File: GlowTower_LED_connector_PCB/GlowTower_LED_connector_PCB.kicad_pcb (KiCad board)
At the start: 2 copper layers, 27 x 27 mm, 8 parts, among them U1 LED strip, U2 LED strip, U3 LED strip, U4 LED strip

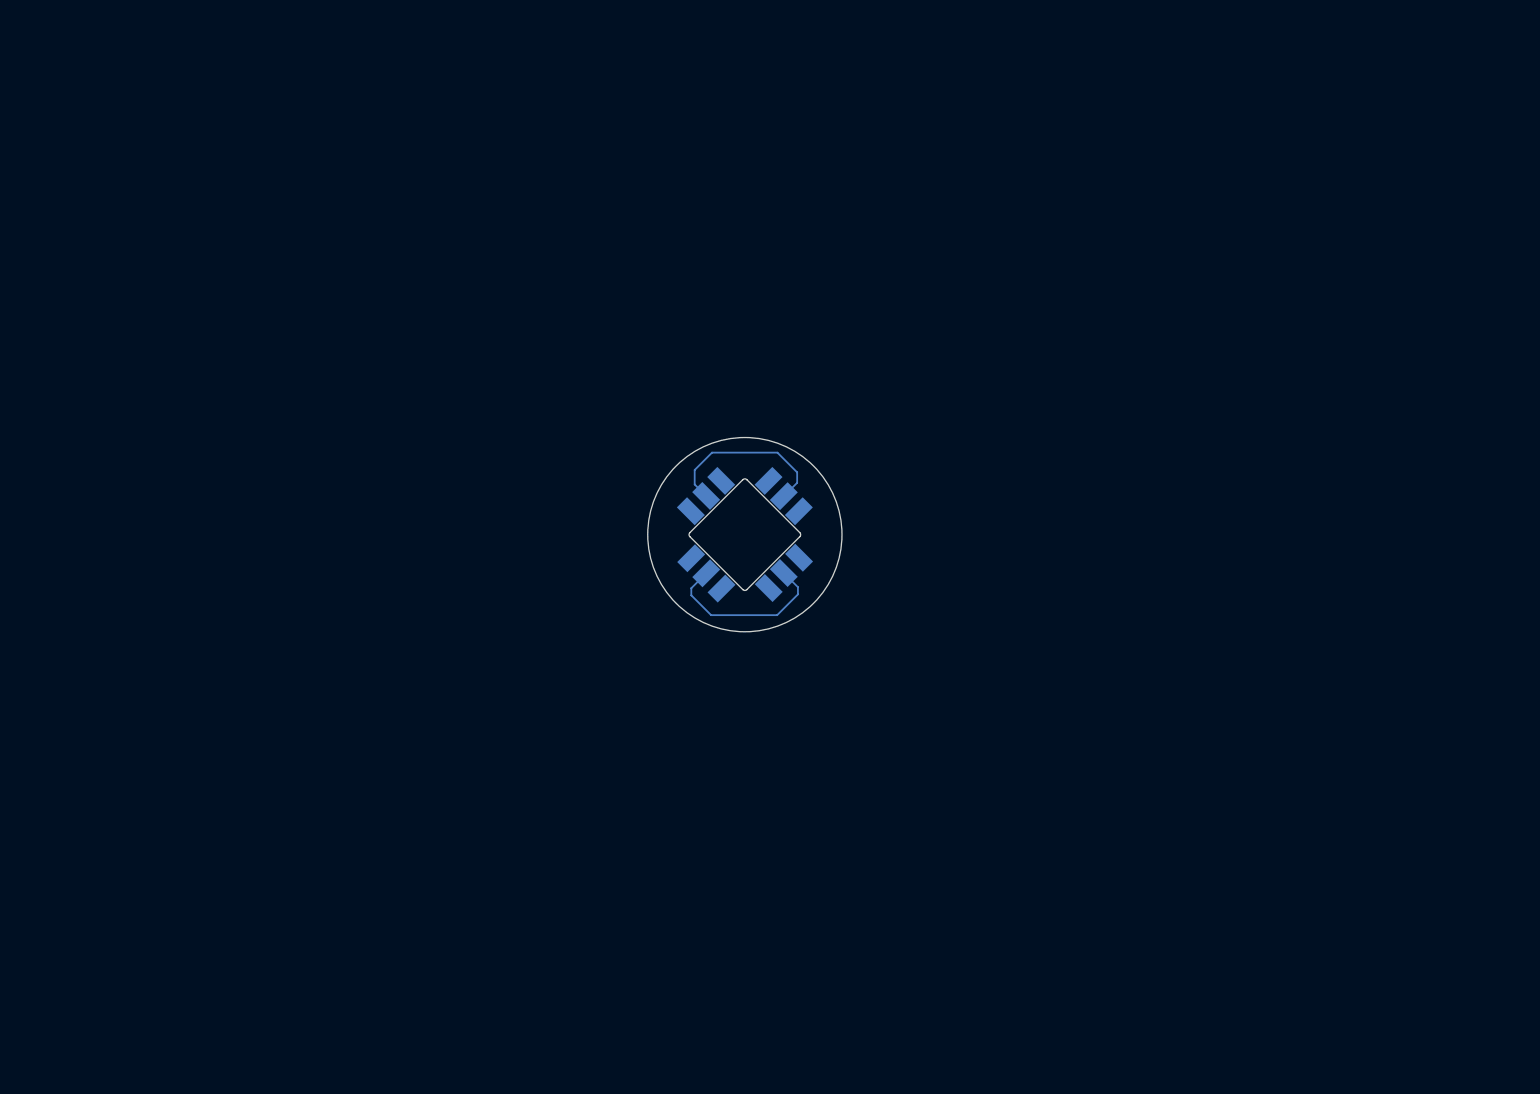
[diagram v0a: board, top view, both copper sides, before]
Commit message: updated pcb design (in progress)
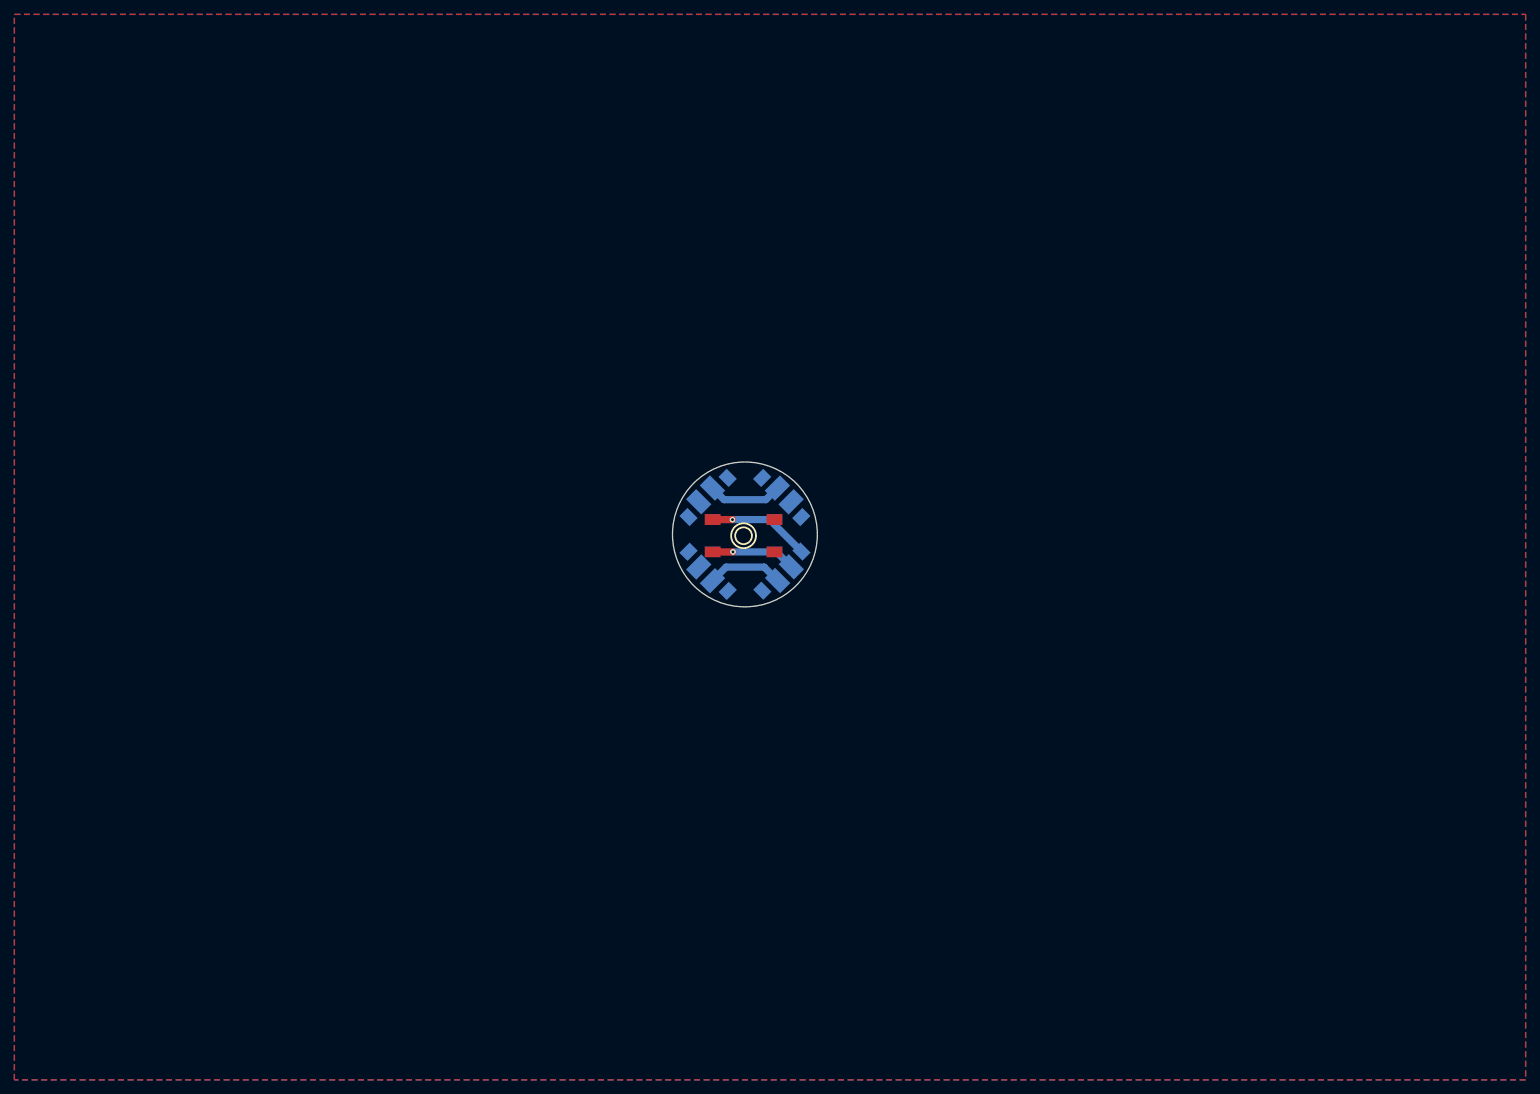
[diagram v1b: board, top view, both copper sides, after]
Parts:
- added SW1: TS-1102S-C-A-B, TS-1102S-C-A-B:TS-1102S-C-A-B, F.Cu at (101.4, 72.4)
- U1, U2, U3, U4: footprint Connector:LED strip connector pad -> myparts:LED strip connector 4pad supersmall
- moved leddirectionarrow1 8.40 mm to (101.5, 66.7)
- moved leddirectionarrow4 8.22 mm to (107.2, 72.0)
- moved leddirectionarrow2 8.12 mm to (96.2, 72.3)
- moved leddirectionarrow3 8.04 mm to (101.7, 77.8)
- moved U3 1.16 mm to (96.8, 77.0)
- moved U1 1.14 mm to (106.5, 77.0)
- moved U2 1.12 mm to (96.8, 67.3)
- moved U4 1.10 mm to (106.4, 67.3)
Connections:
- U1 pad 1: unconnected-(U1-Pad1) -> BUTTON
- U1 pad 2: Net-(U1-Pad2) -> GND
- U1 pad 3: unconnected-(U1-Pad3) -> Net-(U1-Pad3)
- U2 pad 2: Net-(U2-Pad2) -> unconnected-(U2-Pad2)
- U2 pad 3: unconnected-(U2-Pad3) -> Net-(U2-Pad3)
- U3 pad 2: Net-(U1-Pad2) -> Net-(U1-Pad3)
- U4 pad 2: Net-(U2-Pad2) -> Net-(U2-Pad3)
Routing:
- net Net-(U1-Pad2): track 24.9 -> 0.00 mm
- net Net-(U2-Pad2): track 24.7 -> 0.00 mm
- net BUTTON: track 0.00 -> 14.2 mm, vias 0 -> 1
- net GND: track 0.00 -> 11.3 mm, vias 0 -> 1
- net Net-(U1-Pad3): track 0.00 -> 9.61 mm
- net Net-(U2-Pad3): track 0.00 -> 9.38 mm
- added copper zone on B.Cu, net GND
- added copper zone on F.Cu, net GND
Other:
- board size 27 x 27 mm -> 20.1 x 20.1 mm
- board text added: "GlowTower /GlowLight"
- board text added: "LED connector beta 2"
